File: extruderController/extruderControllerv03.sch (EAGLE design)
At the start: 76 parts, among them IC1 LM1117MPX-5.0, IC2 MAX3467CPA, IC3 ATMEGA2561-16AU, IC4 ULN2003AD, J8 615016137621, Q2 PH7030L, Q3 PH7030L, Q4 PH7030L, Q5 PH7030L, Q6 PH7030L, X1 22-23-2081, X2 22-23-2081, X3 22-23-2101, X4 22-23-2051, X5 TSW-102-07-G-D, X8 22-23-2031, X9 22-23-2031

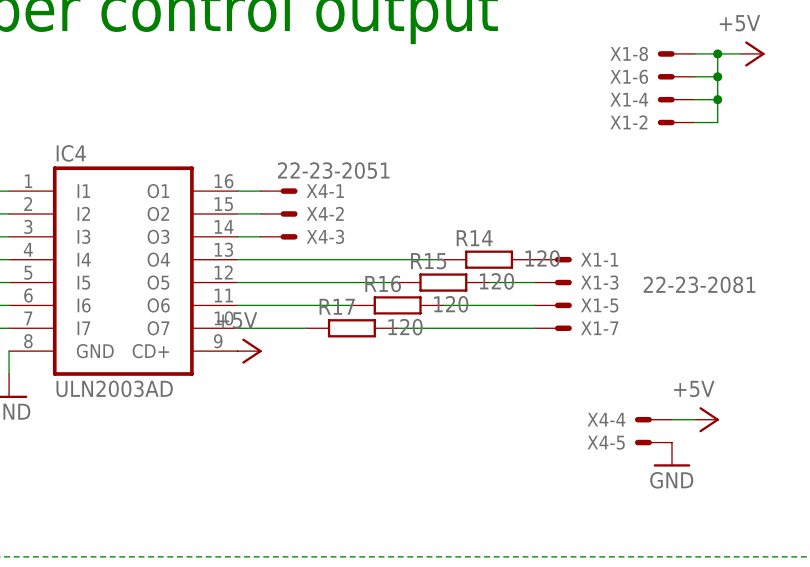
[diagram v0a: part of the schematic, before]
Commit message: g
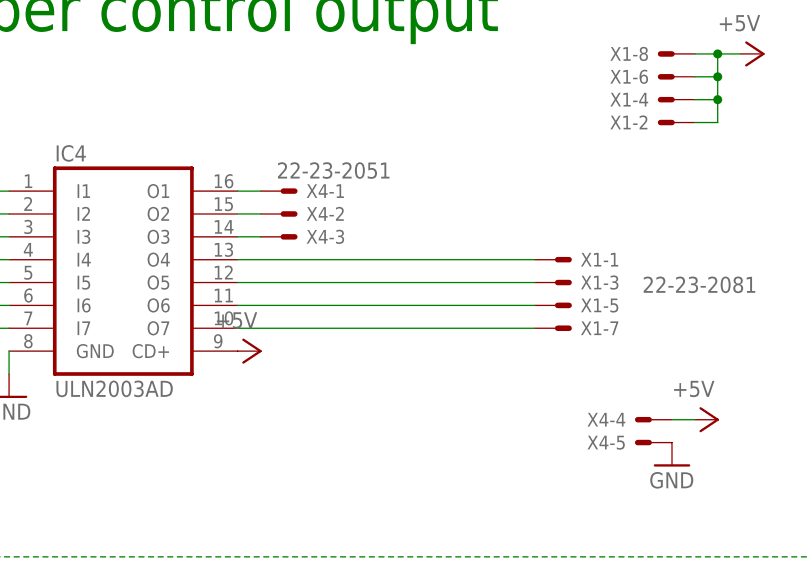
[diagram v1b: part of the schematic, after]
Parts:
- removed R14, R15, R16, R17: 120, rcl:R-EU_R0805
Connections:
- removed net N$3: R14.2, X1-1.S
- removed net N$38: IC4.O5, R15.1
- removed net N$39: IC4.O6, R16.1
- removed net N$40: IC4.O7, R17.1
- net N$12: now also IC4.O5; no longer R15.2
- net N$13: now also IC4.O6; no longer R16.2
- net N$14: now also IC4.O7; no longer R17.2
- net N$30: now also X1-1.S; no longer R14.1
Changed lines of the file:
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@@
 <part name="X8" library="con-molex" library_urn="urn:adsk.eagle:library:165" deviceset="22-23-2031" device=""/>
 <part name="X9" library="con-molex" library_urn="urn:adsk.eagle:library:165" deviceset="22-23-2031" device=""/>
-<part name="R14" library="rcl" library_urn="urn:adsk.eagle:library:334" deviceset="R-EU_" device="R0805" package3d_urn="urn:adsk.eagle:package:23553/2" value="120"/>
-<part name="R15" library="rcl" library_urn="urn:adsk.eagle:library:334" deviceset="R-EU_" device="R0805" package3d_urn="urn:adsk.eagle:package:23553/2" value="120"/>
-<part name="R16" library="rcl" library_urn="urn:adsk.eagle:library:334" deviceset="R-EU_" device="R0805" package3d_urn="urn:adsk.eagle:package:23553/2" value="120"/>
-<part name="R17" library="rcl" library_urn="urn:adsk.eagle:library:334" deviceset="R-EU_" device="R0805" package3d_urn="urn:adsk.eagle:package:23553/2" value="120"/>
 <part name="C13" library="rcl" library_urn="urn:adsk.eagle:library:334" deviceset="C-EU" device="C0603" package3d_urn="urn:adsk.eagle:package:23616/2" value="0.1uF"/>
 <part name="GND8" library="supply1" library_urn="urn:adsk.eagle:library:371" deviceset="GND" device=""/>
@@
 <attribute name="NAME" x="101.6" y="59.182" size="1.524" layer="95" rot="R180"/>
 </instance>
-<instance part="R14" gate="G$1" x="-157.48" y="185.42" smashed="yes">
-<attribute name="NAME" x="-161.29" y="186.9186" size="1.778" layer="95"/>
-<attribute name="VALUE" x="-153.67" y="184.658" size="1.778" layer="96"/>
-</instance>
-<instance part="R15" gate="G$1" x="-162.56" y="182.88" smashed="yes">
-<attribute name="NAME" x="-166.37" y="184.3786" size="1.778" layer="95"/>
-<attribute name="VALUE" x="-158.75" y="182.118" size="1.778" layer="96"/>
-</instance>
-<instance part="R16" gate="G$1" x="-167.64" y="180.34" smashed="yes">
-<attribute name="NAME" x="-171.45" y="181.8386" size="1.778" layer="95"/>
-<attribute name="VALUE" x="-163.83" y="179.578" size="1.778" layer="96"/>
-</instance>
-<instance part="R17" gate="G$1" x="-172.72" y="177.8" smashed="yes">
-<attribute name="NAME" x="-176.53" y="179.2986" size="1.778" layer="95"/>
-<attribute name="VALUE" x="-168.91" y="177.038" size="1.778" layer="96"/>
-</instance>
 <instance part="C13" gate="G$1" x="-86.36" y="93.98" smashed="yes">
 <attribute name="NAME" x="-84.836" y="94.361" size="1.778" layer="95"/>
@@
 </segment>
 </net>
-<net name="N$3" class="0">
-<segment>
-<pinref part="R14" gate="G$1" pin="2"/>
+<net name="N$12" class="0">
+<segment>
+<pinref part="X1" gate="-3" pin="S"/>
+<pinref part="IC4" gate="A" pin="O5"/>
+<wire x1="-152.4" y1="182.88" x2="-185.42" y2="182.88" width="0.1524" layer="91"/>
+</segment>
+</net>
+<net name="N$13" class="0">
+<segment>
+<pinref part="X1" gate="-5" pin="S"/>
+<pinref part="IC4" gate="A" pin="O6"/>
+<wire x1="-185.42" y1="180.34" x2="-152.4" y2="180.34" width="0.1524" layer="91"/>
+</segment>
+</net>
+<net name="N$14" class="0">
+<segment>
+<pinref part="X1" gate="-7" pin="S"/>
+<pinref part="IC4" gate="A" pin="O7"/>
+<wire x1="-152.4" y1="177.8" x2="-185.42" y2="177.8" width="0.1524" layer="91"/>
+</segment>
+</net>
+<net name="N$30" class="0">
+<segment>
+<pinref part="IC4" gate="A" pin="O4"/>
+<wire x1="-185.42" y1="185.42" x2="-152.4" y2="185.42" width="0.1524" layer="91"/>
 <pinref part="X1" gate="-1" pin="S"/>
 </segment>
 </net>
-<net name="N$12" class="0">
-<segment>
-<pinref part="R15" gate="G$1" pin="2"/>
-<pinref part="X1" gate="-3" pin="S"/>
-<wire x1="-152.4" y1="182.88" x2="-157.48" y2="182.88" width="0.1524" layer="91"/>
-</segment>
-</net>
-<net name="N$13" class="0">
-<segment>
-<pinref part="R16" gate="G$1" pin="2"/>
-<pinref part="X1" gate="-5" pin="S"/>
-<wire x1="-152.4" y1="180.34" x2="-162.56" y2="180.34" width="0.1524" layer="91"/>
-</segment>
-</net>
-<net name="N$14" class="0">
-<segment>
-<pinref part="R17" gate="G$1" pin="2"/>
-<pinref part="X1" gate="-7" pin="S"/>
-<wire x1="-152.4" y1="177.8" x2="-167.64" y2="177.8" width="0.1524" layer="91"/>
-</segment>
-</net>
-<net name="N$30" class="0">
-<segment>
-<pinref part="IC4" gate="A" pin="O4"/>
-<pinref part="R14" gate="G$1" pin="1"/>
-<wire x1="-185.42" y1="185.42" x2="-162.56" y2="185.42" width="0.1524" layer="91"/>
-</segment>
-</net>
-<net name="N$38" class="0">
-<segment>
-<pinref part="R15" gate="G$1" pin="1"/>
-<pinref part="IC4" gate="A" pin="O5"/>
-<wire x1="-167.64" y1="182.88" x2="-185.42" y2="182.88" width="0.1524" layer="91"/>
-</segment>
-</net>
-<net name="N$39" class="0">
-<segment>
-<pinref part="IC4" gate="A" pin="O6"/>
-<pinref part="R16" gate="G$1" pin="1"/>
-<wire x1="-185.42" y1="180.34" x2="-172.72" y2="180.34" width="0.1524" layer="91"/>
-</segment>
-</net>
-<net name="N$40" class="0">
-<segment>
-<pinref part="R17" gate="G$1" pin="1"/>
-<pinref part="IC4" gate="A" pin="O7"/>
-<wire x1="-177.8" y1="177.8" x2="-185.42" y2="177.8" width="0.1524" layer="91"/>
-</segment>
-</net>
